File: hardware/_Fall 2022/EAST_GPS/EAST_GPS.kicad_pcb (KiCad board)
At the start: 2 copper layers, 76.2 x 66.7 mm, 7 parts, among them J1 Conn_02x09_Odd_Even, U1 GPS-14414, U2 RFM69HCW_Breakout

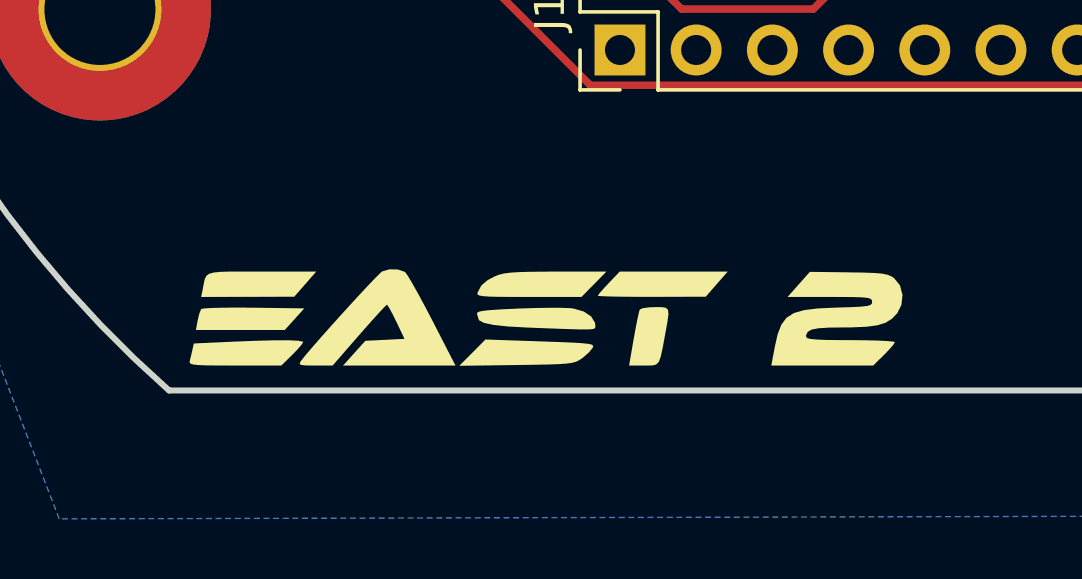
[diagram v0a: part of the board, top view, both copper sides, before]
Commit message: minor fixes
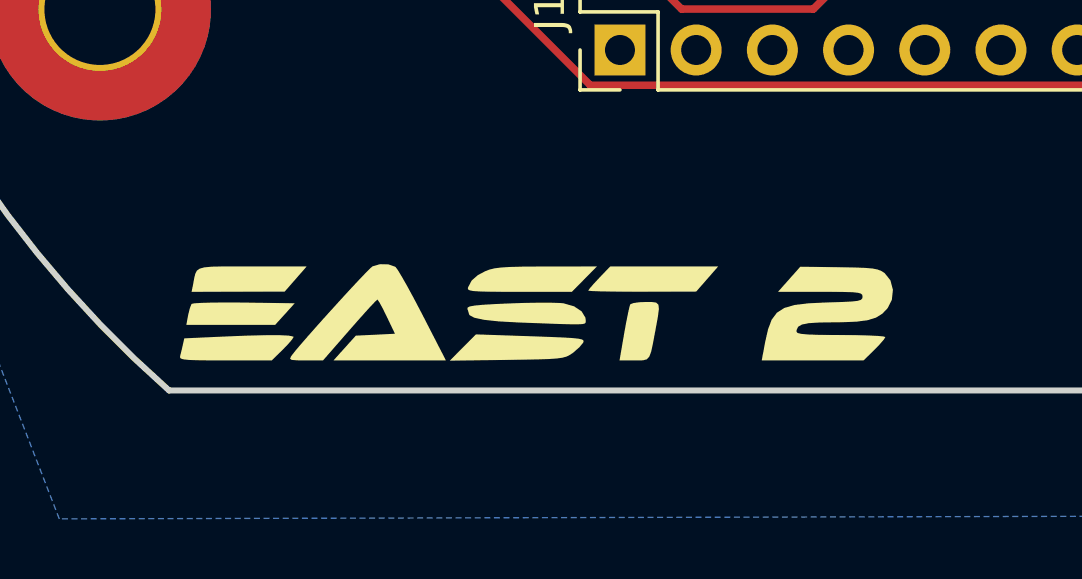
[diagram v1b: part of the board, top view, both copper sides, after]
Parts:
- moved ? 0.36 mm to (130.1, 127.2)
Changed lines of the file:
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@@
   )
   (footprint "LOGO" (layer "F.Cu")
-    (at 130.376838 127.354926)
+    (at 130.05796 127.184274)
     (attr board_only exclude_from_pos_files exclude_from_bom)
     (fp_text reference "" (at 0 0) (layer "F.SilkS")
